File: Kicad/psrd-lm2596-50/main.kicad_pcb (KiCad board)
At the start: 2 copper layers, 150 x 60 mm, 82 parts, among them K1 MAIN AC, K2 PSR1, K3 PSR2, U1 LM2596-50, U2 LM2596-50, X101 LOGO

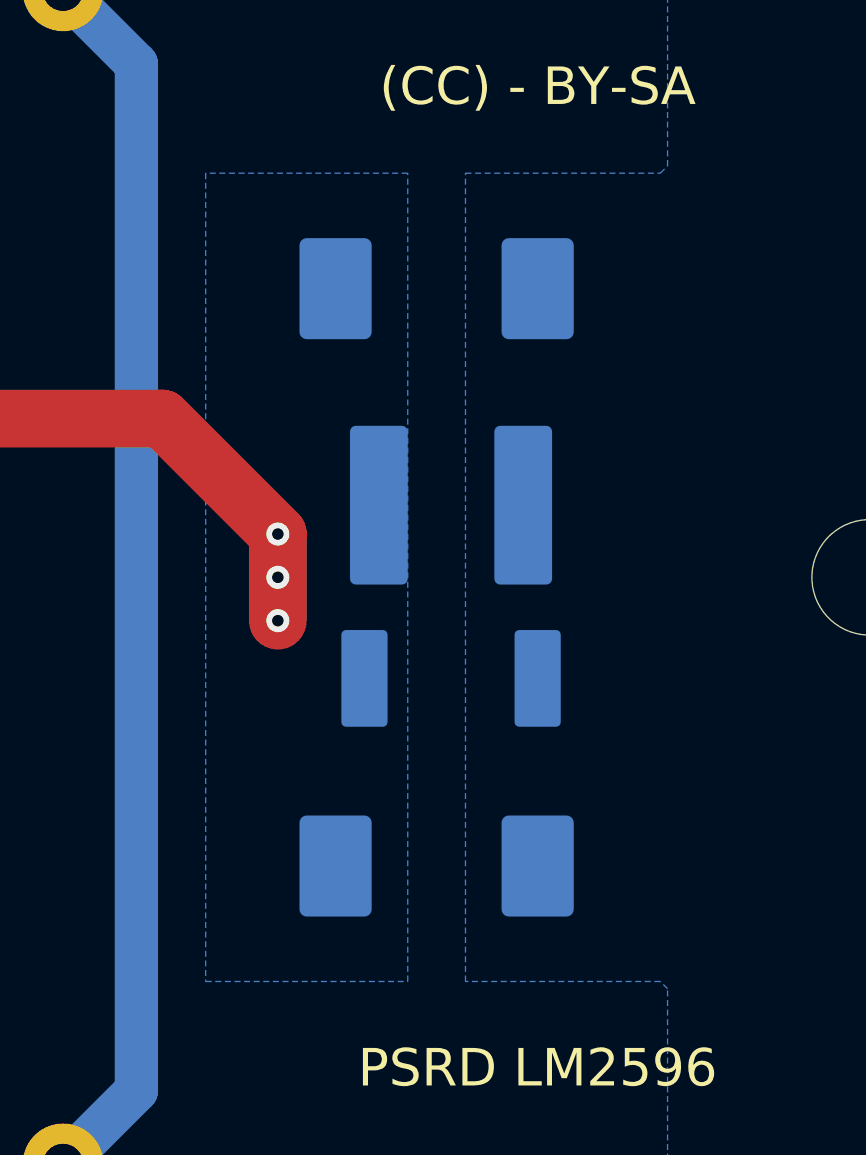
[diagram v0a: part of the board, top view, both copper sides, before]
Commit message: Up
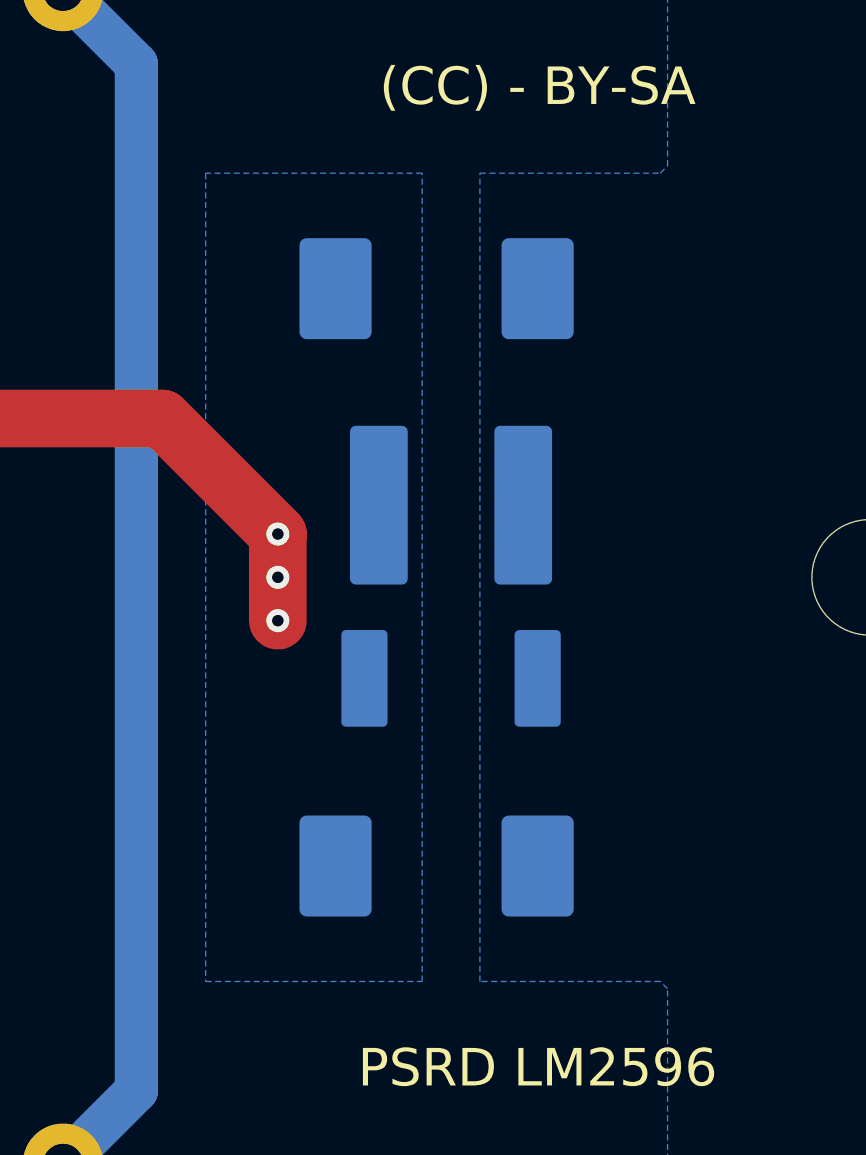
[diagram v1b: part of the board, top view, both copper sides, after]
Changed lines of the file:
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@@
 		(polygon
 			(pts
-				(xy 144.5 98.5) (xy 144.5 109.5) (xy 126 109.5) (xy 126 102.25) (xy 125.750433 102) (xy 119 102)
-				(xy 119 74) (xy 125.75 74) (xy 126 73.75) (xy 126 66.5) (xy 144.5 66.5) (xy 144.5 77.5) (xy 137.25 77.5)
+				(xy 144.5 98.5) (xy 144.5 109.5) (xy 126 109.5) (xy 126 102.25) (xy 125.750433 102) (xy 119.5 102)
+				(xy 119.5 74) (xy 125.75 74) (xy 126 73.75) (xy 126 66.5) (xy 144.5 66.5) (xy 144.5 77.5) (xy 137.25 77.5)
 				(xy 137 77.75) (xy 137 84.250342) (xy 137.25 84.5) (xy 163.5 84.5) (xy 164 84.0002) (xy 164 59.5)
 				(xy 211 59.5) (xy 219 67) (xy 223.5 67) (xy 223.5 109) (xy 219 109) (xy 211 116.5) (xy 164 116.5)
@@
 		(polygon
 			(pts
-				(xy 110 102) (xy 117 102) (xy 117 74) (xy 110 74)
+				(xy 110 102) (xy 117.5 102) (xy 117.5 74) (xy 110 74)
 			)
 		)

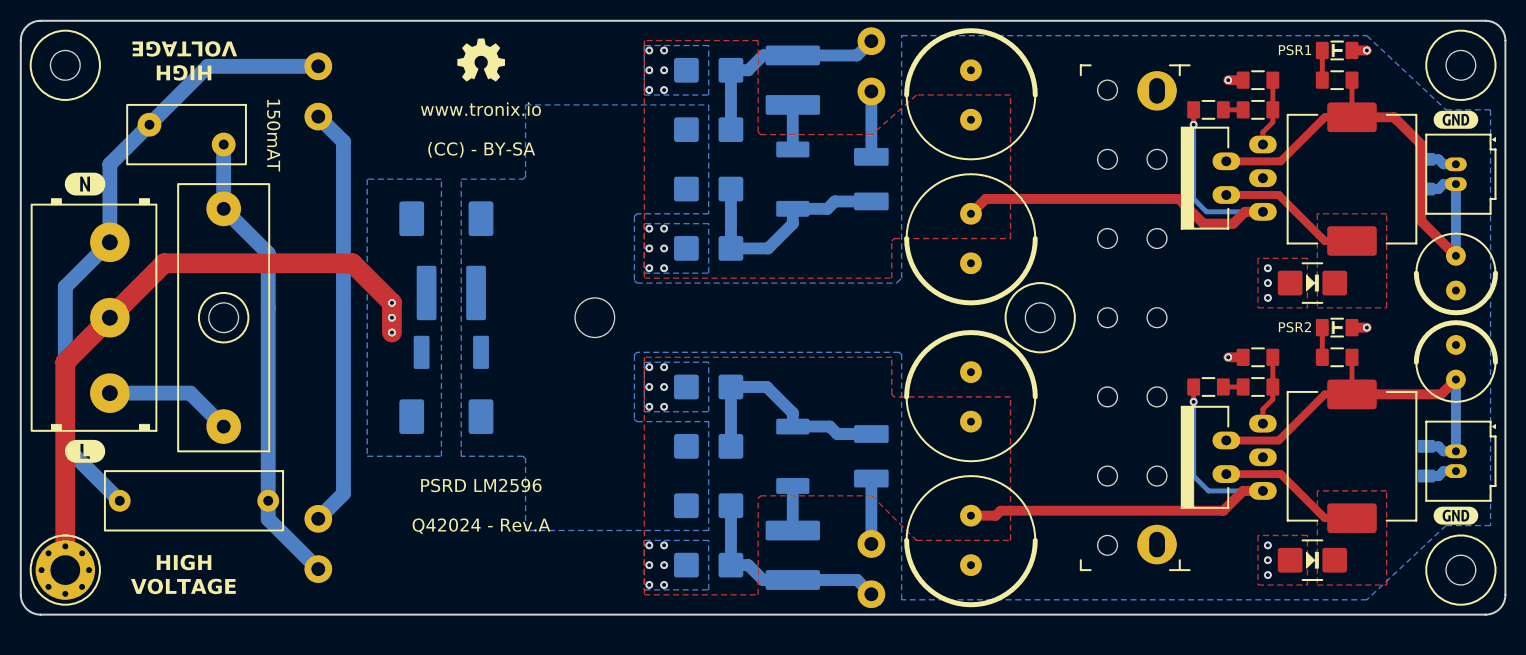
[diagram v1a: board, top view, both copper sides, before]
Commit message: Up
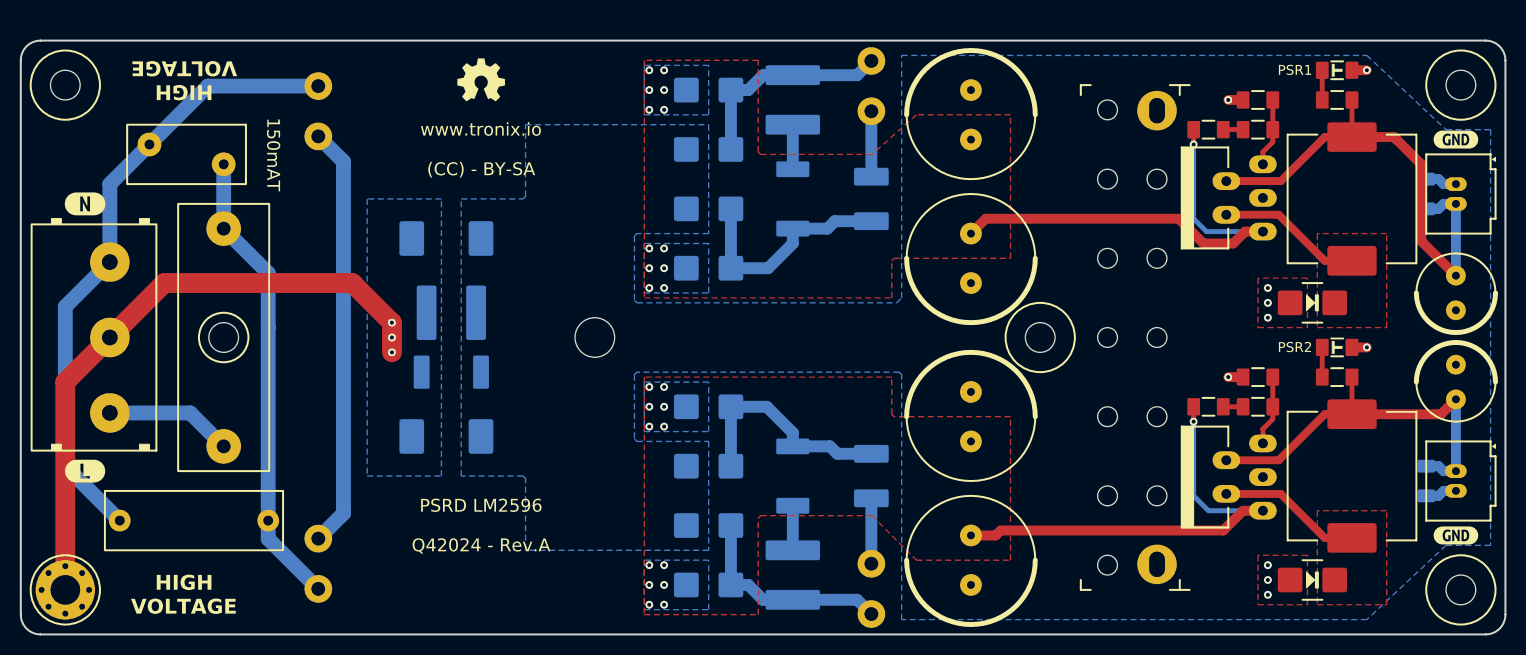
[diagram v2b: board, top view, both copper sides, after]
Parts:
- moved C1 2.00 mm to (92.5, 108.5)
- moved C10 2.00 mm to (217.0, 75.5)
- moved C11 2.00 mm to (217.0, 104.5)
- moved C12 2.00 mm to (220.0, 85.5)
- moved C13 2.00 mm to (220.0, 94.5)
- moved C14 2.00 mm to (118.5, 87.5)
- moved C2 2.00 mm to (153.0, 66.0)
- moved C3 2.00 mm to (153.0, 114.0)
- moved C4 2.00 mm to (171.0, 67.5)
- moved C5 2.00 mm to (171.0, 112.5)
- moved C6 2.00 mm to (171.0, 82.0)
- moved C7 2.00 mm to (171.0, 98.0)
- moved C8 2.00 mm to (195.0, 69.0)
- moved C9 2.00 mm to (195.0, 97.0)
- moved D1 2.00 mm to (144.5, 83.0)
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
